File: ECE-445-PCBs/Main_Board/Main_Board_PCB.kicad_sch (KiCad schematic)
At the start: 39 parts, among them J1 USB_C_Receptacle_USB2.0_16P, J2 Screw_Terminal_01x08, J3 Conn_01x02_Pin, SW1 SW_Push, SW2 SW_Push, U1 ESP32-S3-WROOM-1, U2 TLV62569DDC

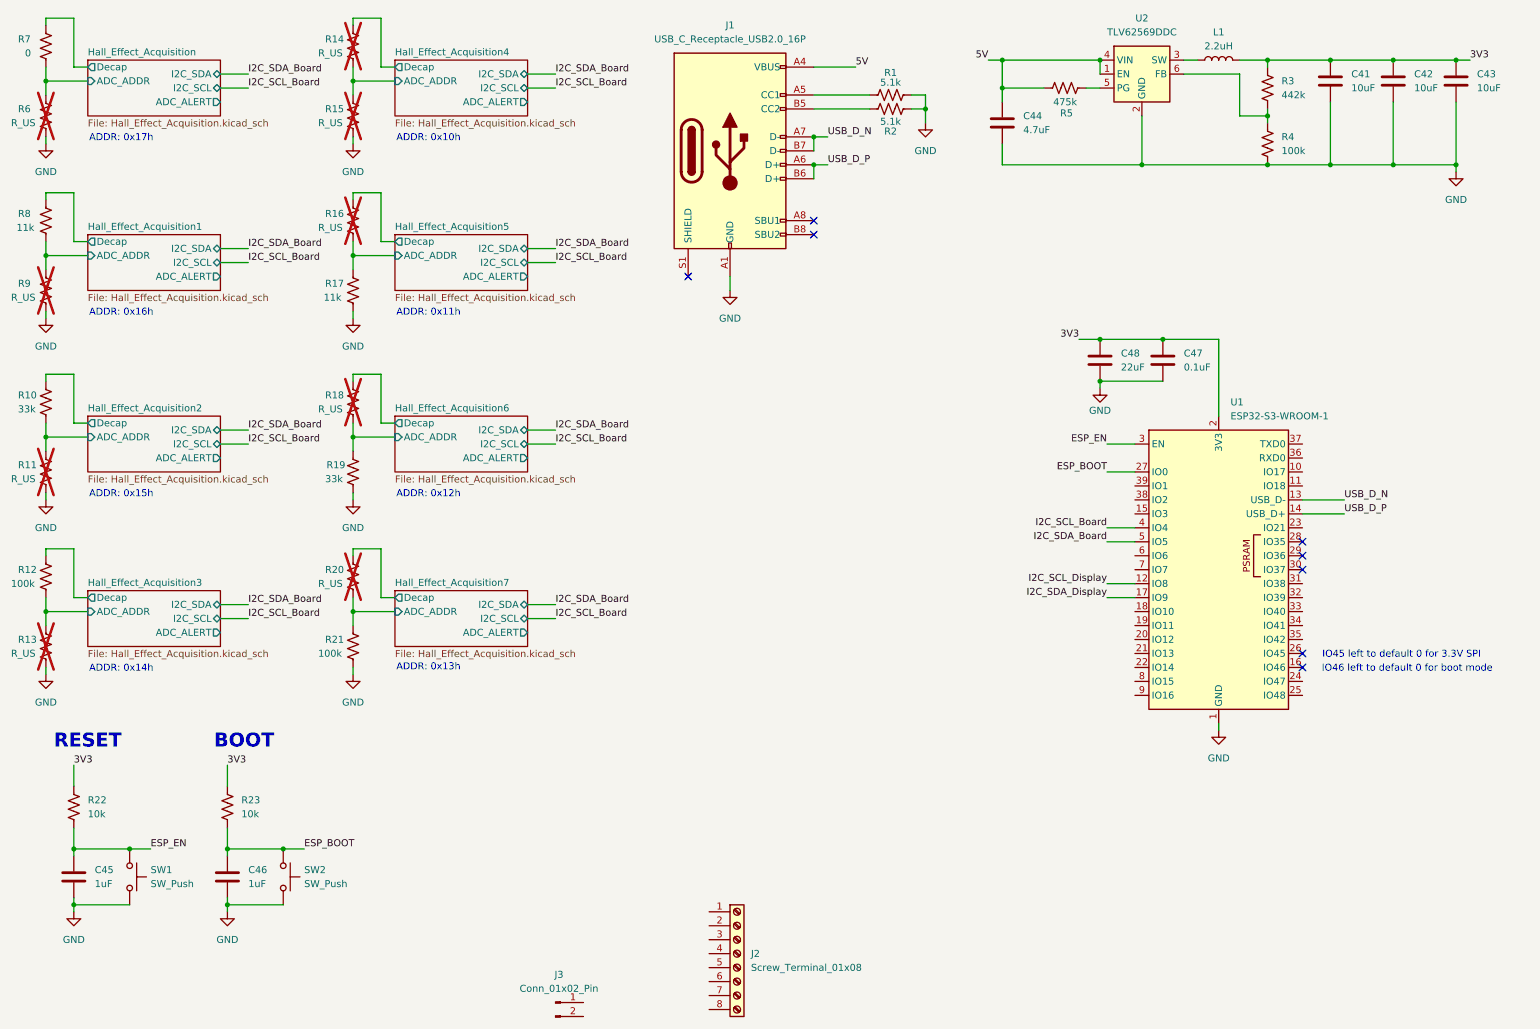
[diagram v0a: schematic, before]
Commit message: started placement
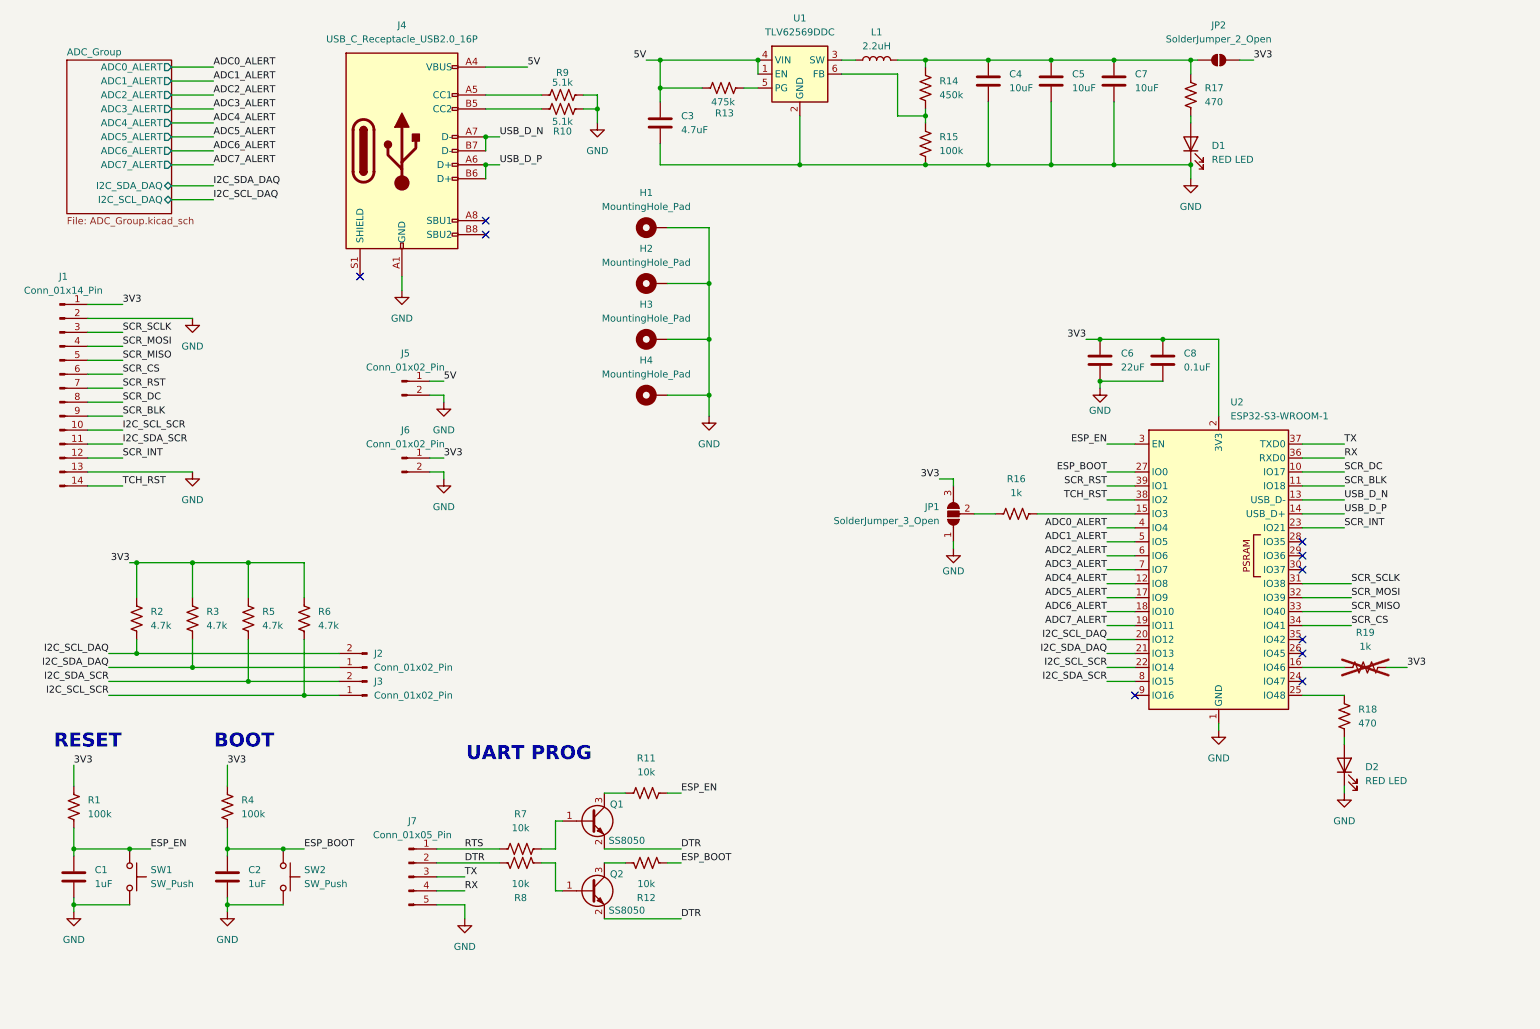
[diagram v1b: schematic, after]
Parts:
- removed J2: Screw_Terminal_01x08, TerminalBlock:OSTVN08A150, symbol Connector:Screw_Terminal_01x08
- removed R10: 33k, symbol Device:R_US
- removed R13, R14, R15, R20, R9: R_US, symbol Device:R_US
- removed R21: 100k, symbol Device:R_US
- added D1, D2: RED LED, LED_SMD:LED_0603_1608Metric, symbol Device:LED
- added H1, H2, H3, H4: MountingHole_Pad, MountingHole:MountingHole_3.2mm_M3_DIN965_Pad, symbol Mechanical:MountingHole_Pad
- added J1: Conn_01x14_Pin, Connector_PinHeader_2.54mm:PinHeader_1x14_P2.54mm_Vertical, symbol Connector:Conn_01x14_Pin
- added J2, J5, J6: Conn_01x02_Pin, Connector_PinHeader_2.54mm:PinHeader_1x02_P2.54mm_Vertical, symbol Connector:Conn_01x02_Pin
- added J7: Conn_01x05_Pin, Connector_PinHeader_2.54mm:PinHeader_1x05_P2.54mm_Vertical, symbol Connector:Conn_01x05_Pin
- added JP1: SolderJumper_3_Open, Jumper:SolderJumper-3_P1.3mm_Open_Pad1.0x1.5mm, symbol Jumper:SolderJumper_3_Open
- added JP2: SolderJumper_2_Open, Jumper:SolderJumper-2_P1.3mm_Open_Pad1.0x1.5mm, symbol Jumper:SolderJumper_2_Open
- added Q1, Q2: SS8050, Package_TO_SOT_SMD:SOT-23, symbol Transistor_BJT:SS8050
- added R2, R3, R5: 4.7k, Resistor_SMD:R_0603_1608Metric, symbol Device:R_US
- C1: renamed from C45; footprint (none) -> Capacitor_SMD:C_0603_1608Metric
- C2: renamed from C46; footprint (none) -> Capacitor_SMD:C_0603_1608Metric
- C3: renamed from C44; footprint (none) -> Capacitor_SMD:C_0603_1608Metric
- C4: renamed from C41; footprint (none) -> Capacitor_SMD:C_0603_1608Metric
- C5: renamed from C42; footprint (none) -> Capacitor_SMD:C_0603_1608Metric
- C6: renamed from C48; footprint (none) -> Capacitor_SMD:C_0603_1608Metric
- C7: renamed from C43; footprint (none) -> Capacitor_SMD:C_0603_1608Metric
- C8: renamed from C47; footprint (none) -> Capacitor_SMD:C_0603_1608Metric
- J3: footprint Connector_Harwin:HARWIN_M20-9990246 -> Connector_PinHeader_2.54mm:PinHeader_1x02_P2.54mm_Vertical
- L1: footprint (none) -> Inductor_SMD:L_Coilcraft_1008HQ_2520Metric
- R1: renamed from R22; value 10k -> 100k; footprint (none) -> Resistor_SMD:R_0603_1608Metric
- R10: renamed from R2; footprint (none) -> Resistor_SMD:R_0603_1608Metric
- R11: value R_US -> 10k; footprint (none) -> Resistor_SMD:R_0603_1608Metric; now fitted
- R12: value 100k -> 10k; footprint (none) -> Resistor_SMD:R_0603_1608Metric
- R13: renamed from R5; footprint (none) -> Resistor_SMD:R_0603_1608Metric
- R14: renamed from R3; value 442k -> 450k; footprint (none) -> Resistor_SMD:R_0603_1608Metric
- R15: renamed from R4; footprint (none) -> Resistor_SMD:R_0603_1608Metric
- R16: value R_US -> 1k; footprint (none) -> Resistor_SMD:R_0603_1608Metric; now fitted
- R17: value 11k -> 470; footprint (none) -> Resistor_SMD:R_0603_1608Metric
- R18: value R_US -> 470; footprint (none) -> Resistor_SMD:R_0603_1608Metric; now fitted
- R19: value 33k -> 1k; footprint (none) -> Resistor_SMD:R_0603_1608Metric; now not fitted
- R4: renamed from R23; value 10k -> 100k; footprint (none) -> Resistor_SMD:R_0603_1608Metric
- R6: value R_US -> 4.7k; footprint (none) -> Resistor_SMD:R_0603_1608Metric; now fitted
- R7: value 0 -> 10k; footprint (none) -> Resistor_SMD:R_0603_1608Metric
- R8: value 11k -> 10k; footprint (none) -> Resistor_SMD:R_0603_1608Metric
- R9: renamed from R1; footprint (none) -> Resistor_SMD:R_0603_1608Metric
- SW1, SW2: footprint (none) -> Button_Switch_THT:SW_TH_Tactile_Omron_B3F-100x
- renumbered J1 to J4, U2 to U1, U1 to U2
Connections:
- net Hall_Effect_Acquisition3/ADC_ADDR is gone; now on net ESP_BOOT: R12.2
- net Hall_Effect_Acquisition6/Decap is gone; now on an unnamed net: R18.1
- net 3V3: now also R19.2, R6.2, J1.1 (Pin_1), J6.1 (Pin_1), JP1.3 (B), JP2.2 (B), R2.2, R3.2, R5.2; no longer C4.2, C5.2, C7.2, L1.2, R14.1
- net 5V: now also J5.1 (Pin_1)
- net ESP_EN: now also R11.2
- net GND: now also D1.1 (K), D2.1 (K), H1.1, H2.1, H3.1, H4.1, J1.13 (Pin_13), J1.2 (Pin_2), J5.2 (Pin_2), J6.2 (Pin_2), J7.5 (Pin_5), JP1.1 (A); no longer R11.2, R17.2, R19.2, R6.2
- net SCR_DC: now reaches U2.10 (IO17)
- net SCR_DC: now also J1.8 (Pin_8)
- net SCR_BLK: now reaches U2.11 (IO18)
- net SCR_BLK: now also J1.9 (Pin_9)
- net at U2.15 (IO3): now also R16.2
- net at U2.16 (IO46): now also R19.1
- net ADC6_ALERT: now reaches U2.18 (IO10)
- net ADC7_ALERT: now reaches U2.19 (IO11)
- net I2C_SCL_DAQ: now reaches U2.20 (IO12)
- net I2C_SCL_DAQ: now also J2.2 (Pin_2), R2.1
- net I2C_SDA_DAQ: now reaches U2.21 (IO13)
- net I2C_SDA_DAQ: now also J2.1 (Pin_1), R3.1
- net I2C_SCL_SCR: now reaches U2.22 (IO14)
- net I2C_SCL_SCR: now also J3.1 (Pin_1), R6.1, J1.10 (Pin_10)
- net SCR_INT: now reaches U2.23 (IO21)
- net SCR_INT: now also J1.12 (Pin_12)
- net SCR_SCLK: now reaches U2.31 (IO38)
- net SCR_SCLK: now also J1.3 (Pin_3)
- net SCR_MOSI: now reaches U2.32 (IO39)
- net SCR_MOSI: now also J1.4 (Pin_4)
- net SCR_MISO: now reaches U2.33 (IO40)
- net SCR_MISO: now also J1.5 (Pin_5)
- net SCR_CS: now reaches U2.34 (IO41)
- net SCR_CS: now also J1.6 (Pin_6)
- net RX: now reaches U2.36 (RXD0)
- net RX: now also J7.4 (Pin_4)
- net TX: now reaches U2.37 (TXD0)
- net TX: now also J7.3 (Pin_3)
- net TCH_RST: now reaches U2.38 (IO2)
- net TCH_RST: now also J1.14 (Pin_14)
- net SCR_RST: now reaches U2.39 (IO1)
- net SCR_RST: now also J1.7 (Pin_7)
- net ADC2_ALERT: now reaches U2.6 (IO6)
- net ADC3_ALERT: now reaches U2.7 (IO7)
- net I2C_SDA_SCR: now reaches U2.8 (IO15)
- net I2C_SDA_SCR: now also J3.2 (Pin_2), J1.11 (Pin_11), R5.1
- net Hall_Effect_Acquisition/ADC_ADDR: no longer names the net of R7.2
- net Hall_Effect_Acquisition/ADC_ADDR: now also Q1.1 (B); no longer R6.1
- net Hall_Effect_Acquisition/Decap renamed RTS
- net RTS: now also J7.1 (Pin_1)
- net Hall_Effect_Acquisition1/ADC_ADDR: no longer names the net of R8.2
- net Hall_Effect_Acquisition1/ADC_ADDR: now also Q2.1 (B)
- net Hall_Effect_Acquisition1/Decap renamed DTR
- net DTR: now also J7.2 (Pin_2), Q1.2 (E), Q2.2 (E)
- net Hall_Effect_Acquisition2/ADC_ADDR: no longer names the net of R11.1
- net Hall_Effect_Acquisition2/ADC_ADDR: now also Q1.3 (C)
- net Hall_Effect_Acquisition3/Decap: no longer names the net of R12.1
- net Hall_Effect_Acquisition3/Decap: now also Q2.3 (C)
- net Hall_Effect_Acquisition5/ADC_ADDR: no longer names the net of R17.1
- net Hall_Effect_Acquisition5/ADC_ADDR: now also C4.2, C5.2, C7.2, L1.2, R14.1, JP2.1 (A); no longer R16.2
- net Hall_Effect_Acquisition5/Decap: no longer names the net of R16.1
- net Hall_Effect_Acquisition5/Decap: now also JP1.2 (C)
- net Hall_Effect_Acquisition6/ADC_ADDR: no longer names the net of R18.2
- net Hall_Effect_Acquisition6/ADC_ADDR: now also D2.2 (A); no longer R19.1
- net I2C_SCL_Board renamed ADC0_ALERT
- net I2C_SCL_Display renamed ADC4_ALERT
- net I2C_SDA_Board renamed ADC1_ALERT
- net I2C_SDA_Display renamed ADC5_ALERT
- new net: D1.2 (A), R17.2
- no-connect marks 8 -> 10
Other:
- removed sheet Hall_Effect_Acquisition
- removed sheet Hall_Effect_Acquisition1
- removed sheet Hall_Effect_Acquisition2
- removed sheet Hall_Effect_Acquisition3
- removed sheet Hall_Effect_Acquisition4
- removed sheet Hall_Effect_Acquisition5
- removed sheet Hall_Effect_Acquisition6
- removed sheet Hall_Effect_Acquisition7
- added sheet ADC_Group (ADC_Group.kicad_sch)
- note added: "UART PROG"
- note removed: "ADDR: 0x10h"
- note removed: "ADDR: 0x11h"
- note removed: "ADDR: 0x12h"
- note removed: "ADDR: 0x13h"
- note removed: "ADDR: 0x14h"
- note removed: "ADDR: 0x15h"
- note removed: "ADDR: 0x16h"
- note removed: "ADDR: 0x17h"
- note removed: "IO45 left to default 0 for 3.3V SPI"
- note removed: "IO46 left to default 0 for boot mode"
- moved on the sheet: C3, C4, C5, C7, J4, L1, R10, R13, R14, R15, R9, U1
